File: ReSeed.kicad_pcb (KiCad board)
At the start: 2 copper layers, 60.8 x 99.9 mm, 45 parts, among them CN1 EDGE_CONNECTOR, CN2 AUDIO_OUT, CN3 AUDIO_IN, CN4 DB9_MALE, Q1 2SC1815, SW1 SW_DIGIFIX, U1 MOS_8580, U2 CD4520BE, U3 74LS245, U4 GAL16V8, U5 TL497ACN

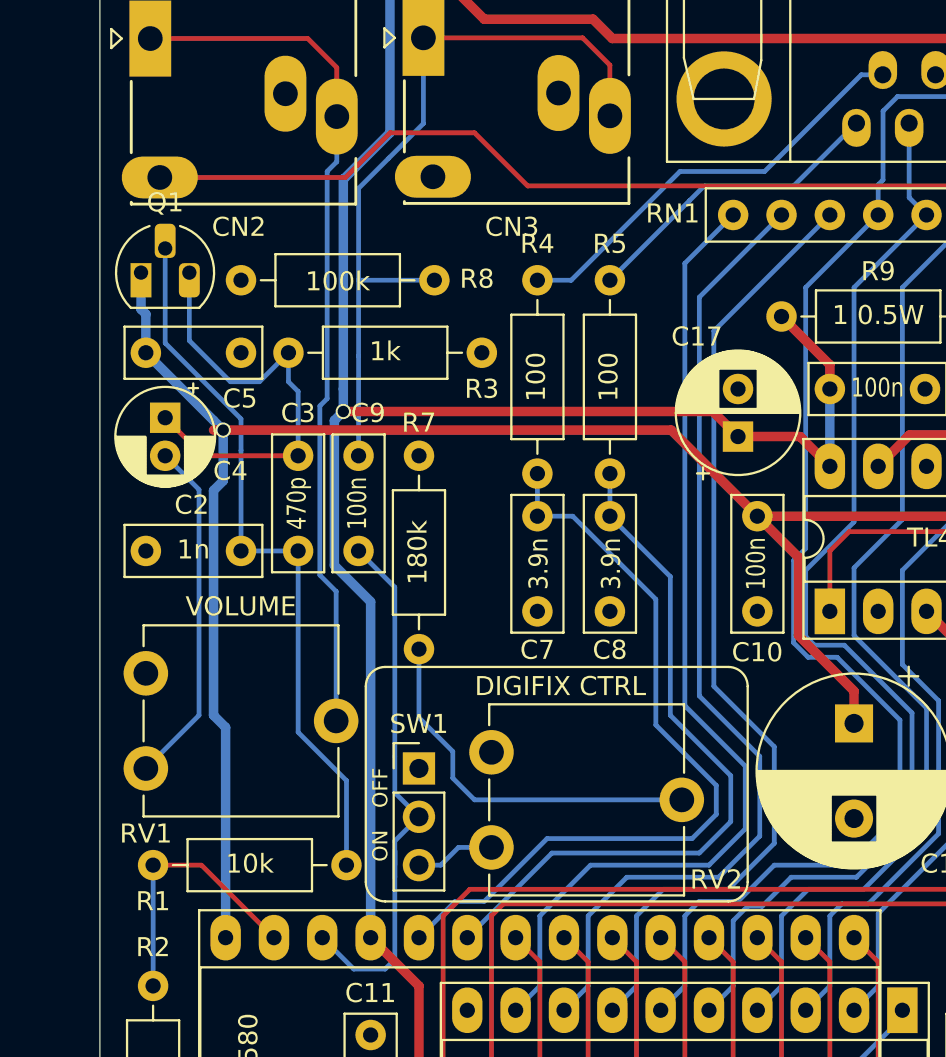
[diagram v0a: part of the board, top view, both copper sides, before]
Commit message: Stehe ich in Flammen
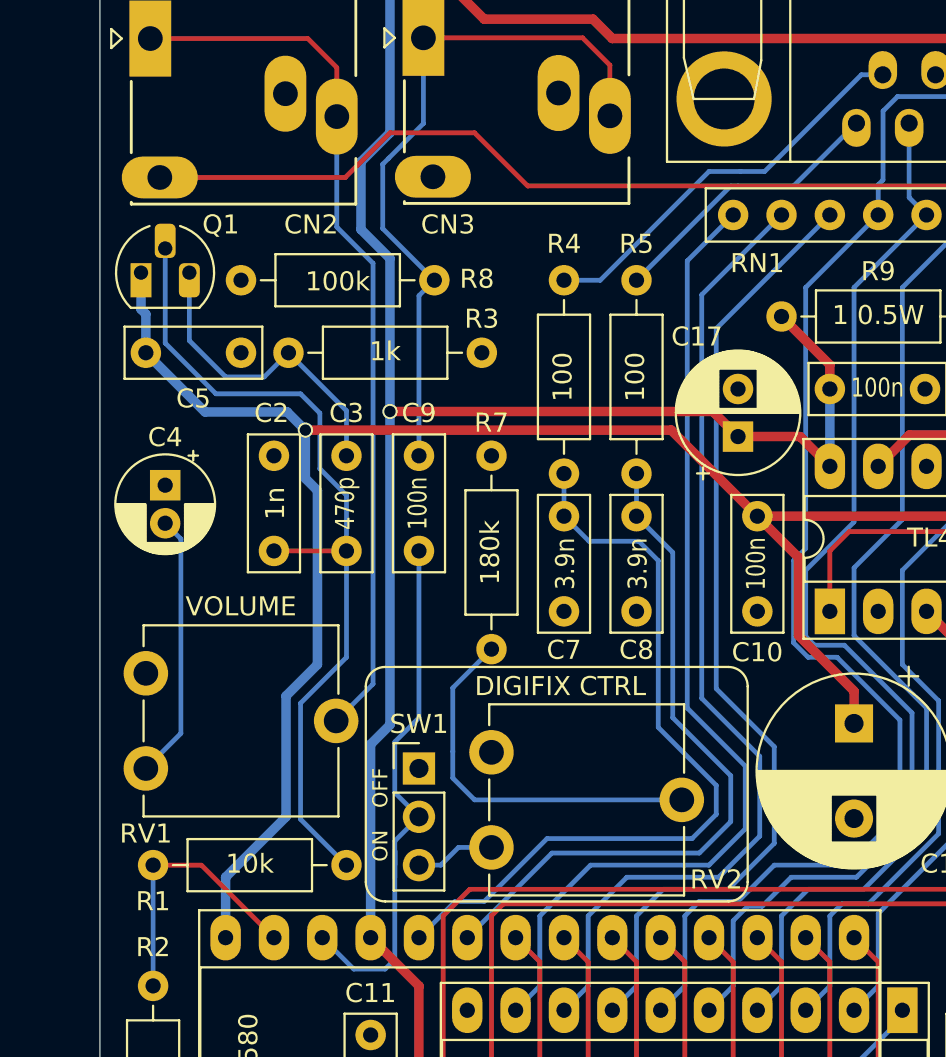
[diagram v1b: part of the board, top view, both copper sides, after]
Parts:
- moved R7 3.81 mm to (142.4, 75.9)
- moved C4 3.54 mm to (125.2, 77.4)
- moved C9 3.17 mm to (138.6, 75.9)
- moved C3 2.54 mm to (134.7, 75.9)
- moved C2 1.73 mm to (130.9, 80.9), turned to 90 degrees
- moved C7 1.40 mm to (146.2, 79.1)
- moved C8 1.40 mm to (150.0, 79.1)
- moved R4 1.40 mm to (146.2, 66.7)
- moved R5 1.40 mm to (150.0, 66.7)
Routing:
- net Net-(C3-Pad1): track 23.7 -> 16.8 mm
- net Net-(C2-Pad1): track 38.1 -> 44.8 mm
- net Net-(C4-Pad2): track 18.3 -> 14.0 mm
- net Net-(C9-Pad1): track 40.4 -> 37.4 mm
- net +5V: track 307.5 -> 304.6 mm
- net /poty: track 16.4 -> 15.0 mm
- net /potx: track 22.6 -> 21.2 mm
- net +9V: track 105.0 -> 106.3 mm
- net Net-(CN2-PadR): track 45.5 -> 46.4 mm
- net Net-(C8-Pad1): track 37.3 -> 36.7 mm
